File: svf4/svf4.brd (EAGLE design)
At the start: 58.4 x 216.8 mm, 79 parts, among them IC1 OPA4130P, IC2 OPA2134P, Q1 BC550B, Q10 2N3906, Q2 BC550B, Q3 2N3904, Q4 2N3904, Q5 2N3904, Q6 2N3904, Q7 2N3906, Q8 2N3906, Q9 2N3906

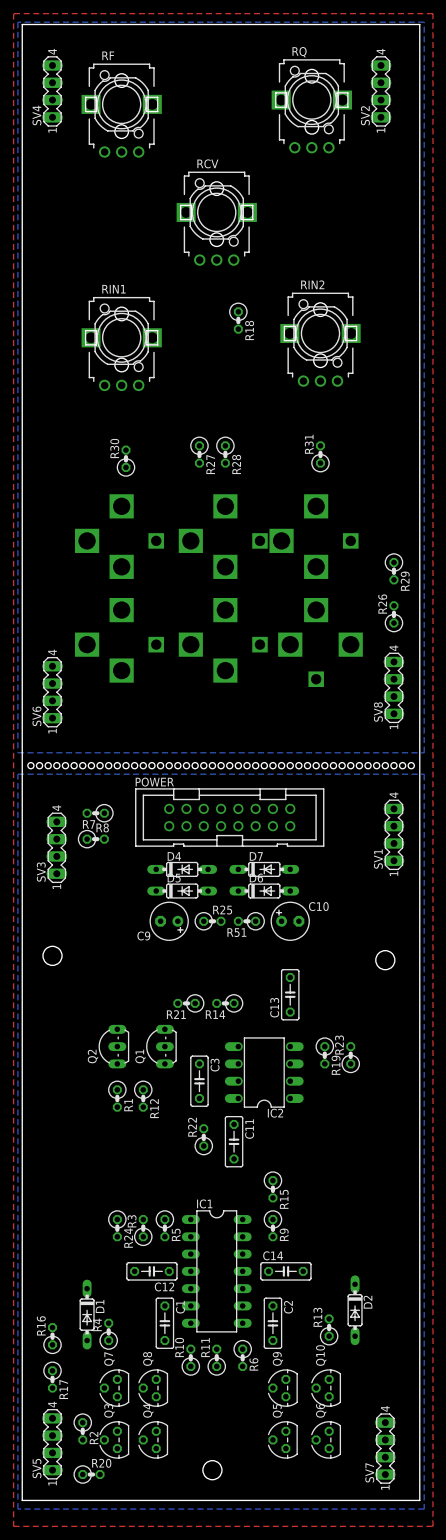
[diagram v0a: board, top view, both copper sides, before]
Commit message: finished the rough draft of the state variable board
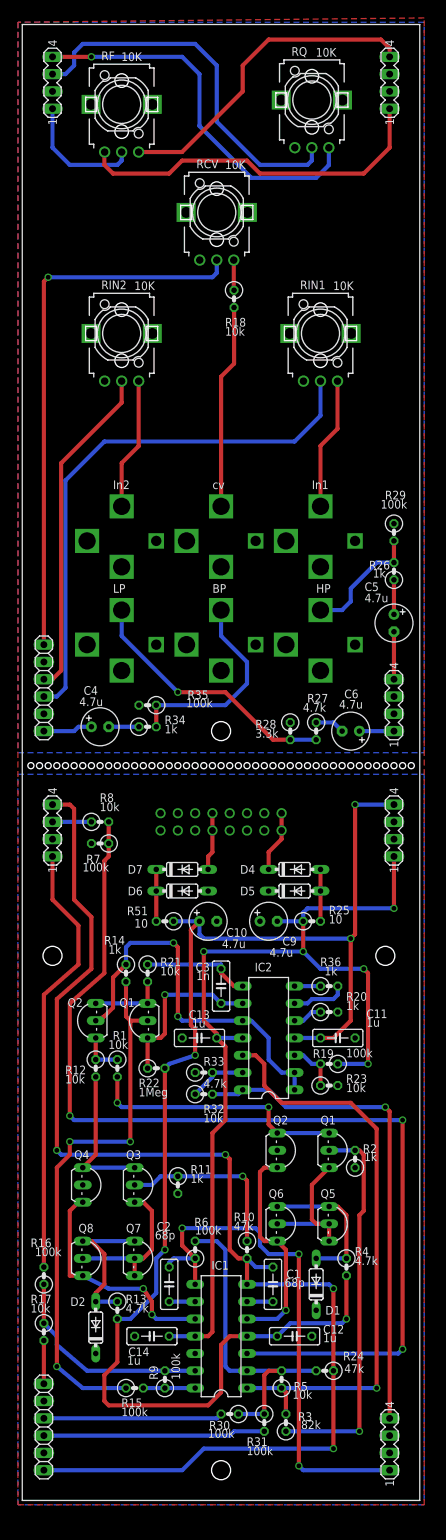
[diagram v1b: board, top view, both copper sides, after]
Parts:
- removed Q10, Q7, Q8, Q9: 2N3906, dan:TO92
- removed Q3, Q4, Q5, Q6: 2N3904, dan:TO92
- removed SV5, SV6: (no value), dan:MA04-1
- added C4, C5, C6: 4.7u, dan:E2,5-6
- added JP1, JP2: (no value), dan:1X06
- added R32: 10k, dan:0207/2V
- added R33: 4.7k, dan:0207/2V
- added R34, R36: 1k, dan:0207/2V
- added R35: 100k, dan:0207/2V
- added U$1, U$2, U$3, U$4: 2N3904_, dan:TO92-EBC
- added U$5, U$6, U$7, U$8: 2N3906_, dan:TO92-EBC
- IC2: value OPA2134P -> OPA4130P; device dan:DIL08 -> dan:DIL14
- R20: value 220k -> 1k
- R27: value 1k -> 4.7k
- R28: value 1k -> 3.3k
- R29: value 1k -> 100k
- R3: value 100k -> 82k
- R30, R31: value 10k -> 100k
- moved R31 142.5 mm to (35.6, 11.4), turned to 270 degrees
- moved R30 141.2 mm to (30.5, 12.7), turned to 180 degrees
- moved R20 76.4 mm to (45.1, 71.8)
- moved R2 56.6 mm to (48.9, 50.2), turned to 90 degrees
- moved R27 44.1 mm to (43.2, 113.0)
- moved R28 41.7 mm to (39.4, 113.0)
- moved D2 38.2 mm to (10.8, 25.4), turned to 90 degrees
- moved R24 37.0 mm to (44.5, 19.1), turned to 180 degrees
- moved R4 36.2 mm to (47.6, 34.3), turned to 270 degrees
- moved R15 35.6 mm to (16.5, 16.5), turned to 0 degrees
- moved R3 35.4 mm to (38.7, 11.4)
- moved D1 33.9 mm to (43.2, 31.8), turned to 90 degrees
- moved R13 31.2 mm to (14.0, 27.9), turned to 270 degrees
- moved RIN1 29.2 mm to (43.8, 171.4)
- moved RIN2 29.2 mm to (14.6, 171.4)
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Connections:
- new net N$38: BPOUT.P$3, R34.2, R35.1
- new net N$41: IC2.14, R32.2, SV7.4
- new net N$42: IC2.13, R32.1, R33.2
- new net N$43: C6.-, R27.1
- new net N$44: C5.+, R26.1
- new net N$45: C4.-, R34.1
- new net N$46: JP2.4, R31.2
- new net N$47: IC2.5, R20.1
- new net N$48: IC2.6, R36.2
- net +12V: now also IC2.4; no longer IC2.8
- net -12V: now also IC2.11; no longer IC2.4
- net -1V: now also IC2.10; no longer IC2.5
- net BP: now also JP2.6; no longer SV5.1
- net GND: now also JP1.2, JP1.5, JP2.2, JP2.5, R20.2, R33.1, R35.2, U$2.B, U$4.B; no longer Q4.2, Q6.2, SV5.2, SV6.2
- net HP: now also IC2.12; no longer SV7.4
- net IN: now also IC1.2, R24.2, R30.1, R31.1, R5.2, R6.2; no longer R20.2, SV5.3
- net N$1: now also U$3.C, U$4.C; no longer Q5.3, Q6.3
- net N$10: now also U$4.E, U$8.E; no longer Q10.1, Q6.1
- net N$14: now also U$3.E, U$7.B, U$7.E, U$8.B; no longer Q10.2, Q5.1, Q9.1, Q9.2
- net N$15: now also U$3.B; no longer Q5.2
- net N$16: now also JP2.1; no longer SV5.4
- net N$17: now also U$7.C, U$8.C; no longer Q10.3, Q9.3
- net N$2: now also U$2.E, U$6.E; no longer Q4.1, Q8.1
- net N$26: now also IC2.8; no longer IC2.7
- net N$28: now also IC2.9; no longer IC2.6
- net N$3: now also U$5.C, U$6.C; no longer Q7.3, Q8.3
- net N$30: now also JP1.1; no longer SV6.4
- net N$32: now also C5.-; no longer R26.1
- net N$33: now also JP1.4; no longer R30.2
- net N$36: now also C4.+, JP1.6; no longer BPOUT.P$3, SV6.1
- net N$37: now also JP2.3, R30.2; no longer R30.1, R31.1, SV6.3
- net N$4: now also U$1.E, U$5.B, U$5.E, U$6.B; no longer Q3.1, Q7.1, Q7.2, Q8.2
- net N$40: now also JP1.3; no longer R31.2
- net N$5: now also U$1.C, U$2.C; no longer Q3.3, Q4.3
- net N$6: now also U$1.B; no longer Q3.2
- net N$7: now also IC2.7, R36.1; no longer IC1.2, R20.1, R24.2, R5.2, R6.2
- net N$8: now also C6.+; no longer R27.1
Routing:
- net +12V: track 0.00 -> 253.6 mm, vias 0 -> 5
- net -12V: track 0.00 -> 195.6 mm, vias 0 -> 5
- net BP: track 0.00 -> 187.8 mm, vias 0 -> 4
- net N$9: track 0.00 -> 151.7 mm, vias 0 -> 3
- net HP: track 0.00 -> 87.2 mm, vias 0 -> 1
- net N$30: track 0.00 -> 81.2 mm, vias 0 -> 1
- net N$33: track 0.00 -> 80.7 mm
- net N$21: track 0.00 -> 80.3 mm, vias 0 -> 3
- net LP: track 0.00 -> 78.3 mm, vias 0 -> 3
- net N$41: track 0.00 -> 72.7 mm, vias 0 -> 1
- net FCIN: track 0.00 -> 64.2 mm
- net N$6: track 0.00 -> 57.0 mm, vias 0 -> 1
- net -1V: track 0.00 -> 56.2 mm, vias 0 -> 2
- net N$25: track 0.00 -> 55.8 mm, vias 0 -> 1
- net N$31: track 0.00 -> 55.4 mm
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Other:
- board size 58.4 x 216.8 mm -> 10.6 x 2.1 mm
- board text added: "-12V"
- board text added: "BP"
- board text added: "HP"
- board text added: "In1"
- board text added: "In2"
- board text added: "LP"
- board text added: "Q1"
- board text added: "Q2"
- board text added: "Q3"
- board text added: "Q4"
- board text added: "Q5"
- board text added: "Q6"
- board text added: "Q7"
- board text added: "Q8"
- board text added: "cv"
